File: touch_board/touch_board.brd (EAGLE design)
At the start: 68.2 x 39.4 mm, 29 parts, among them IC1 PIC18F47K42-I_PT, IC2 MAX203EEWP, X1 RS-232-1, X2 RS-232-2, X3 POWER, X4 22-23-2041

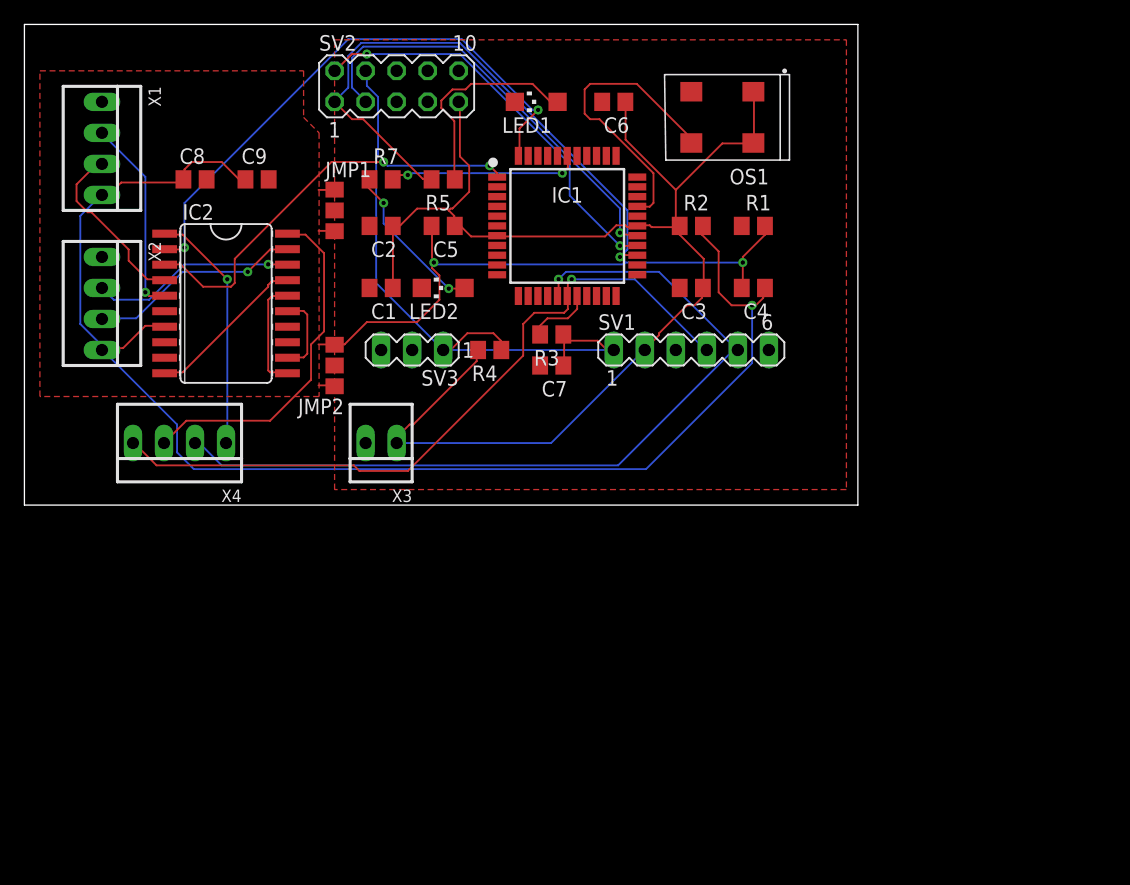
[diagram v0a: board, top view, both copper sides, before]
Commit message: update
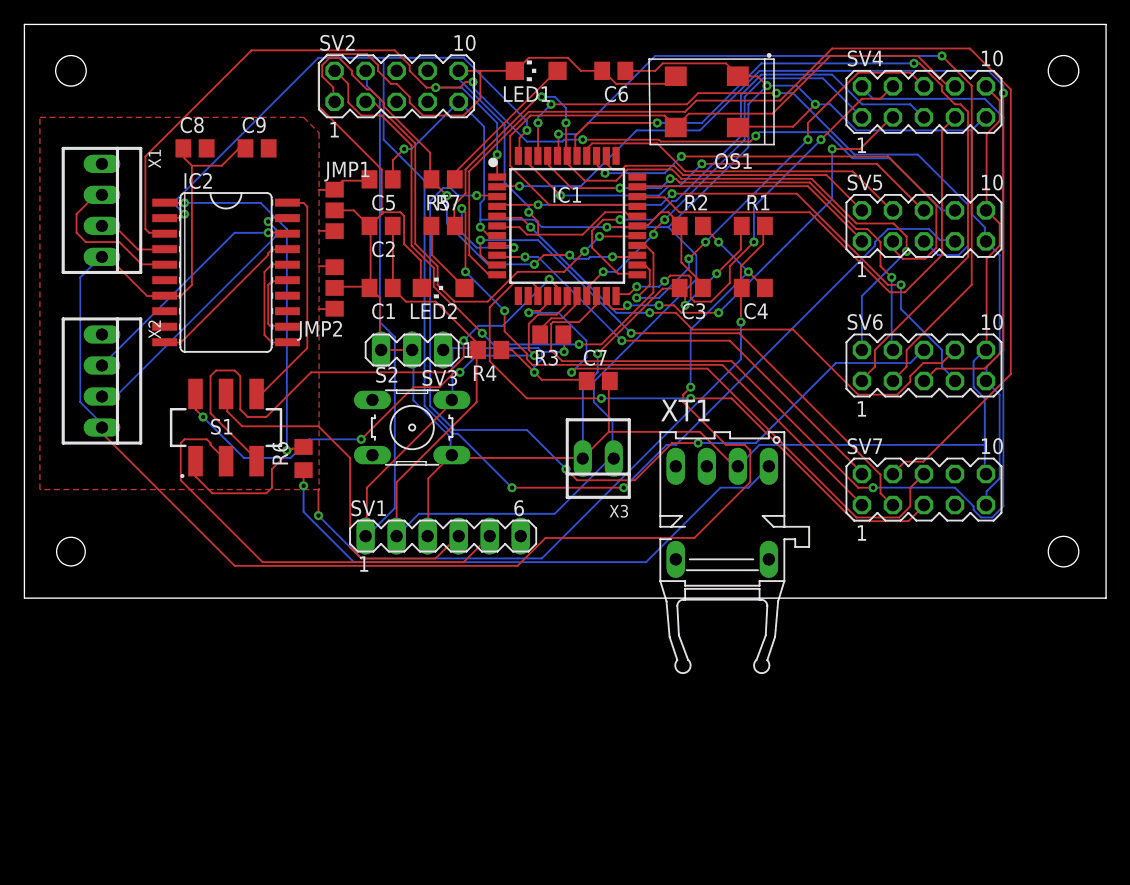
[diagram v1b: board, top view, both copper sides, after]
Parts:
- removed X4: 22-23-2041, con-molex:22-23-2041
- added R6: 220, rcl:R0805
- added S1: ICD/SERIAL, JS202011SCQN:JS202011SCQN
- added S2: RESET_PB, switch-omron:B3F-10XX
- added SV4, SV5, SV6, SV7: IO1, con-lstb:MA05-2
- added XT1: HFBR-1521, fiber-optic-hp:HFBR-15X3
- moved SV1 25.4 mm to (41.9, 38.1)
- moved X3 17.8 mm to (54.6, 44.5)
- moved JMP2 6.35 mm to (33.0, 58.4)
- moved X2 6.35 mm to (14.0, 50.8)
- moved C5 6.35 mm to (36.8, 67.3)
- moved R7 6.35 mm to (41.9, 63.5)
- moved X1 5.08 mm to (14.0, 64.8)
- moved C7 4.02 mm to (54.6, 50.8), turned to 0 degrees
- moved C6 2.54 mm to (55.9, 76.2)
- moved LED1 2.54 mm to (49.5, 76.2)
- moved IC2 2.54 mm to (24.1, 59.7)
- moved C8 2.54 mm to (21.6, 69.8)
- moved C9 2.54 mm to (26.7, 69.8)
- moved OS1 1.80 mm to (63.5, 73.7)
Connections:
- new net N$23: S1.5, SV1.4
- new net N$24: S1.2, SV1.5
- new net N$25: R6.1, XT1.1
- new net N$26: IC1.19, SV4.1
- new net N$27: IC1.20, SV4.2
- new net N$28: IC1.21, SV4.3
- new net N$29: IC1.22, SV4.4
- new net N$30: IC1.23, SV4.5
- new net N$31: IC1.31, SV4.7
- new net N$32: IC1.24, SV4.6
- new net N$33: IC1.32, SV5.1
- new net N$34: IC1.35, SV5.2
- new net N$35: IC1.36, SV5.3
- new net N$36: IC1.37, SV5.4
- new net N$37: IC1.42, SV5.5
- new net N$38: IC1.43, SV5.6
- new net N$39: IC1.38, SV6.1
- new net N$40: IC1.40, SV6.3
- new net N$41: IC1.41, SV6.4
- new net N$42: IC1.2, SV6.5
- new net N$43: IC1.3, SV6.6
- new net N$44: IC1.4, SV6.7
- new net N$45: IC1.5, SV6.8
- new net N$46: IC1.8, SV7.1
- new net N$47: IC1.9, SV7.2
- new net N$48: IC1.10, SV7.3
- new net N$49: IC1.11, SV7.4
- new net N$50: IC1.14, SV7.5
- new net N$51: IC1.15, SV7.6
- net N$1: now also SV4.8
- net N$10: now also SV6.2
- net N$19: now also SV5.7
- net N$2: now also S2.2
- net N$20: now also R6.2, S1.1; no longer X4.1
- net N$21: now also SV5.8
- net N$22: now also S1.4; no longer X4.3
- net N$6: now also S1.6; no longer SV1.4, X4.4
- net N$7: now also S1.3; no longer SV1.5, X4.2
- net VDD: now also SV4.9, SV5.9, SV6.9, SV7.9
- net VSS: now also S2.4, SV4.10, SV5.10, SV6.10, SV7.10, XT1.2
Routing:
- net VSS: track 0.00 -> 242.2 mm, vias 0 -> 4
- net VDD: track 113.2 -> 215.2 mm, vias 0 -> 5
- net N$49: track 0.00 -> 96.1 mm
- net N$27: track 0.00 -> 95.1 mm, vias 0 -> 1
- net N$19: track 46.7 -> 127.5 mm, vias 2 -> 4
- net N$42: track 0.00 -> 75.1 mm, vias 0 -> 2
- net N$43: track 0.00 -> 70.4 mm, vias 0 -> 3
- net N$40: track 0.00 -> 66.2 mm, vias 0 -> 2
- net N$39: track 0.00 -> 63.9 mm, vias 0 -> 2
- net N$21: track 34.1 -> 95.3 mm, vias 2 -> 5
- net N$46: track 0.00 -> 55.1 mm, vias 0 -> 4
- net N$50: track 0.00 -> 51.5 mm, vias 0 -> 2
- net N$37: track 0.00 -> 50.7 mm, vias 0 -> 3
- net N$51: track 0.00 -> 47.6 mm, vias 0 -> 2
- net N$10: track 15.7 -> 62.5 mm, vias 2 -> 3
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- removed copper zone on layer 1, net VSS
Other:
- board size 68.2 x 39.4 mm -> 88.6 x 47 mm

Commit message: update
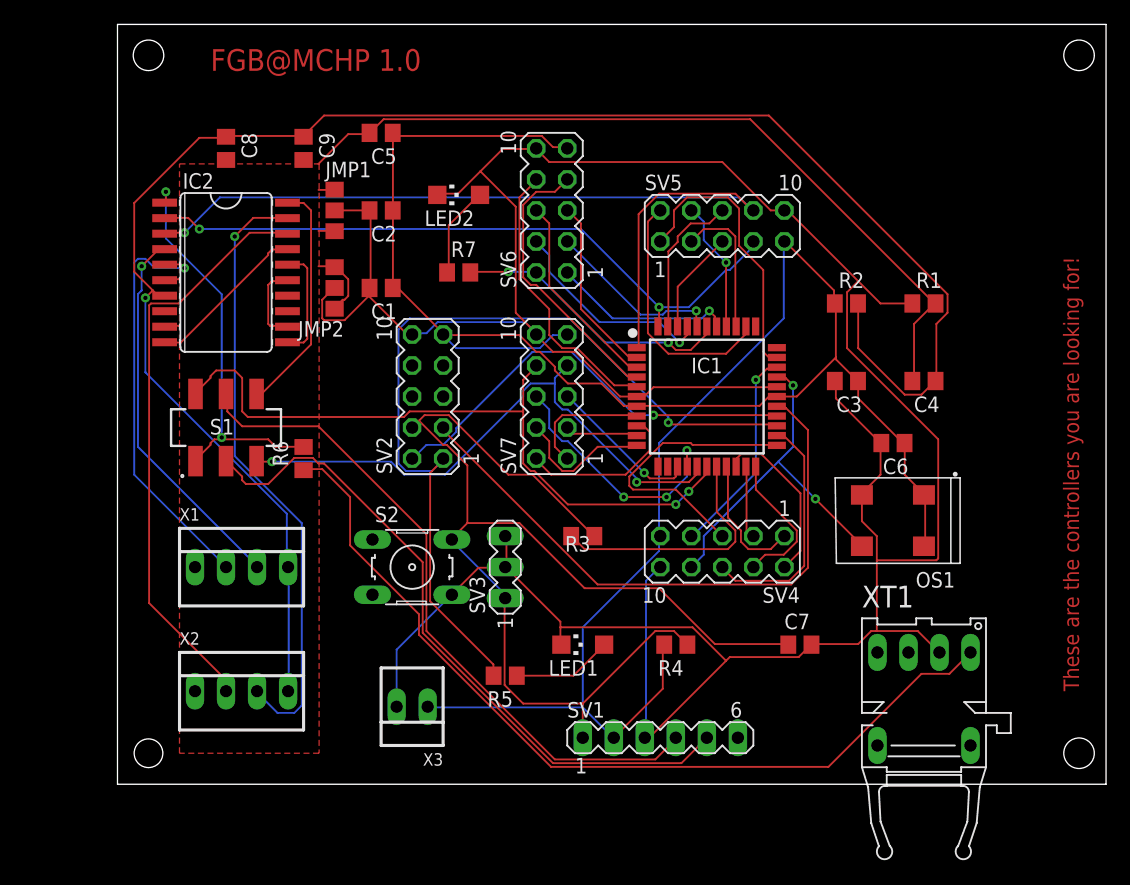
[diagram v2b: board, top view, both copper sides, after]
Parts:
- moved LED1 47.1 mm to (53.3, 29.2)
- moved R5 41.0 mm to (47.0, 26.7)
- moved SV4 40.4 mm to (64.8, 36.8), turned to 180 degrees
- moved C6 38.1 mm to (78.7, 45.7)
- moved OS1 37.5 mm to (78.7, 39.4)
- moved SV6 33.0 mm to (50.8, 64.8), turned to 90 degrees
- moved SV7 31.4 mm to (50.8, 49.5), turned to 90 degrees
- moved X1 31.4 mm to (25.4, 35.6), turned to 0 degrees
- moved R4 28.5 mm to (61.0, 29.2)
- moved X2 27.9 mm to (25.4, 25.4), turned to 0 degrees
- moved C7 27.2 mm to (71.1, 29.2)
- moved SV2 25.5 mm to (40.6, 49.5), turned to 90 degrees
- moved X3 25.4 mm to (39.4, 24.1)
- moved SV1 24.3 mm to (59.7, 21.6)
- moved XT1 22.5 mm to (81.3, 19.1)
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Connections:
- net N$6: now also SV7.8
- net N$7: now also SV7.7
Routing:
- net N$49: track 96.1 -> 11.5 mm
- net N$27: track 95.1 -> 14.0 mm, vias 1 -> 0
- net N$19: track 127.5 -> 55.4 mm, vias 4 -> 2
- net N$42: track 75.1 -> 14.8 mm, vias 2 -> 0
- net N$43: track 70.4 -> 16.6 mm, vias 3 -> 0
- net N$40: track 66.2 -> 14.5 mm, vias 2 -> 1
- net N$39: track 63.9 -> 15.0 mm, vias 2 -> 1
- net N$46: track 55.1 -> 10.4 mm, vias 4 -> 0
- net N$37: track 50.7 -> 8.48 mm, vias 3 -> 0
- net N$48: track 46.6 -> 6.05 mm, vias 2 -> 0
- net N$10: track 62.5 -> 23.3 mm, vias 3 -> 2
- net N$50: track 51.5 -> 12.6 mm, vias 2 -> 1
- net VDD: track 215.2 -> 181.8 mm, vias 5 -> 0
- net N$4: track 40.1 -> 71.1 mm, vias 4 -> 1
- net N$16: track 19.7 -> 48.0 mm, vias 1 -> 0
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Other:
- board size 88.6 x 47 mm -> 81 x 62.2 mm
- board text added: "FGB@MCHP 1.0"
- board text added: "These are the controllers you are looking for!"
